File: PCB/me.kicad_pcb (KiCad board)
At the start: 2 copper layers, 107.9 x 100 mm, 16 parts, among them M1 Motor_DC, Q1 AO3400A, SW1 SW_Push, SW2 SW_Push, SW3 SW_Push, SW4 SW_Push, SW5 SW_Push, SW6 SW_Push, U1 XIAO-RP2040-DIP

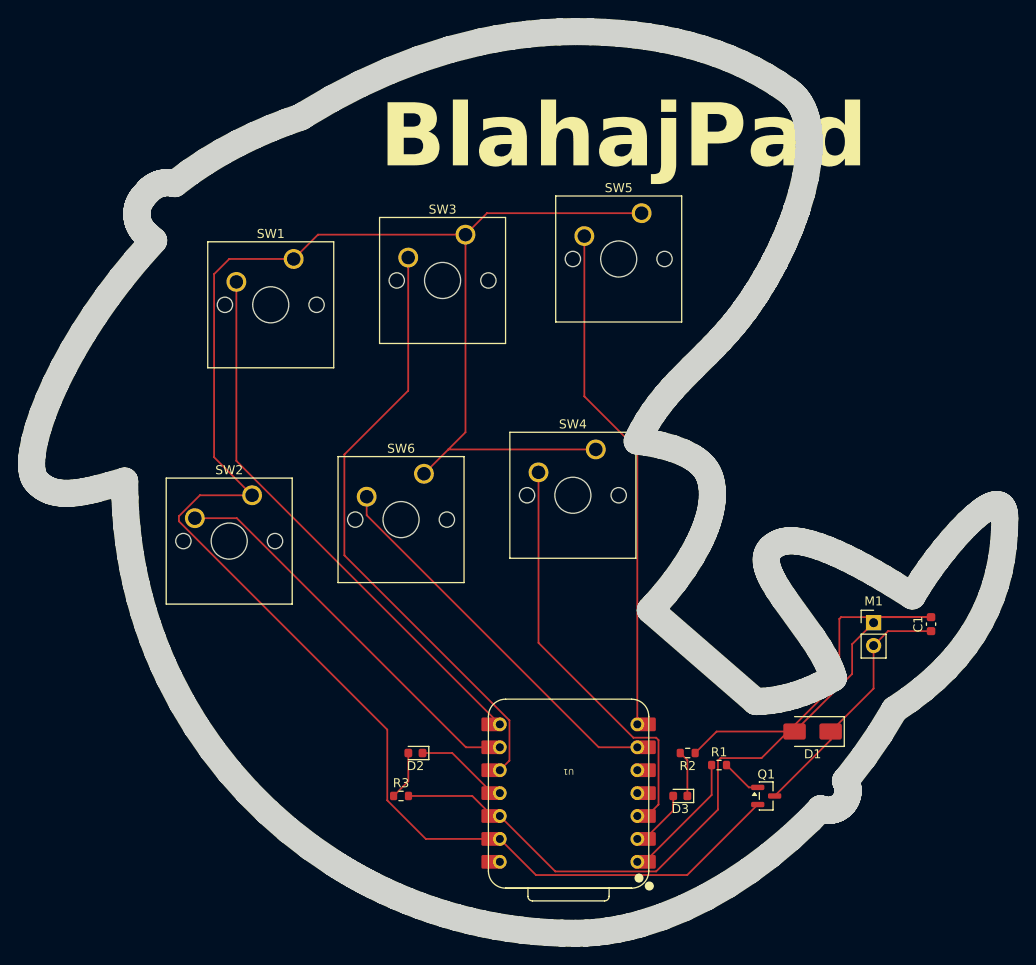
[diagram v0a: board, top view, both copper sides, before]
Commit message: everything's smaller now
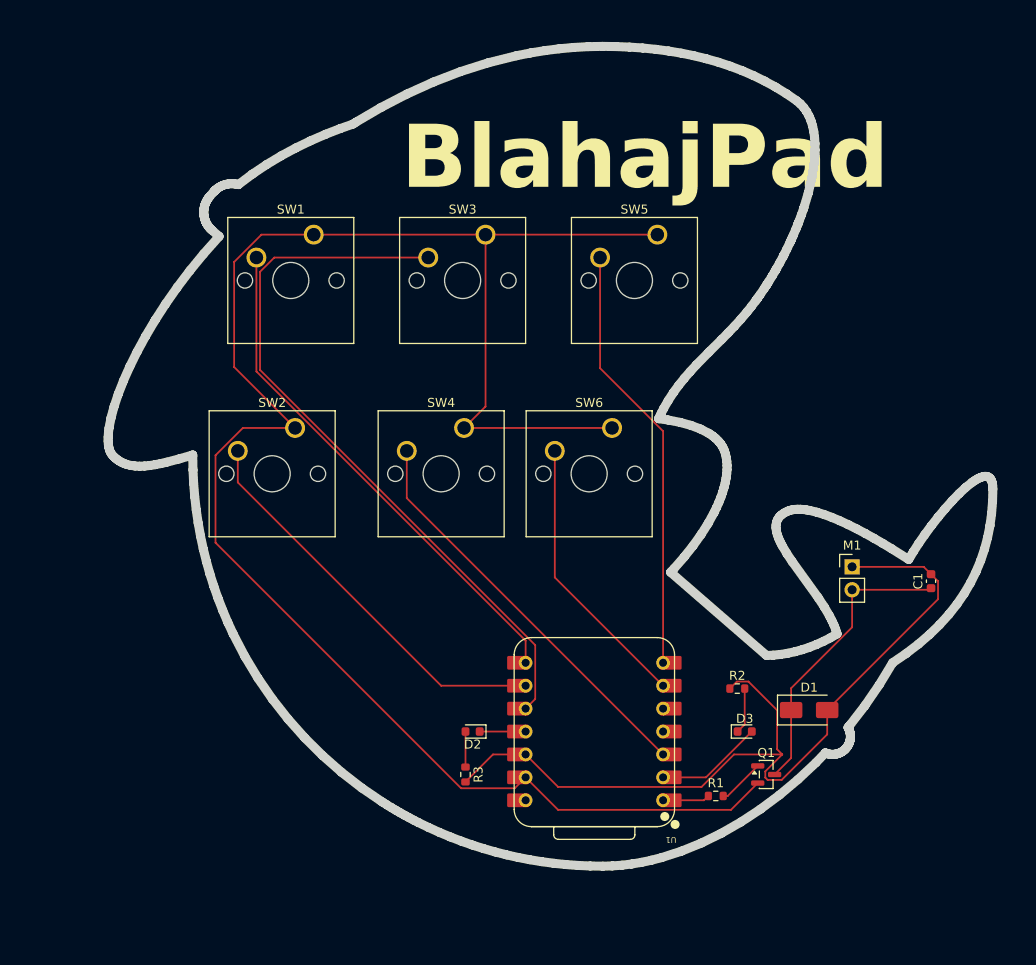
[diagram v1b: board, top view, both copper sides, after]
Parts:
- moved SW6 21.5 mm to (161.5, 92.6)
- moved SW4 14.8 mm to (145.1, 92.6)
- moved D3 10.1 mm to (176.2, 126.2), turned to 0 degrees
- moved R2 9.01 mm to (175.4, 121.4), turned to 0 degrees
- moved SW2 8.85 mm to (126.4, 92.6)
- moved R3 7.53 mm to (145.3, 131.0), turned to -90 degrees
- moved U1 7.40 mm to (159.5, 126.2)
- moved D2 6.77 mm to (146.0, 126.2)
- moved M1 6.63 mm to (188.1, 108.0)
- moved C1 4.76 mm to (196.9, 109.5)
- moved SW1 3.50 mm to (128.4, 71.1)
- moved R1 3.45 mm to (173.0, 133.3)
- moved SW5 2.95 mm to (166.5, 71.1)
- moved D1 2.41 mm to (183.4, 123.8), turned to 0 degrees
- moved Q1 2.38 mm to (178.6, 131.0)
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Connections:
- U1 pad 14: +5V -> unconnected-(U1-VBUS-Pad14)_1
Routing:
- net +3.3V: track 113.7 -> 96.0 mm
- net GND: track 219.1 -> 202.6 mm
- net Net-(U1-GPIO4/MISO): track 68.4 -> 80.8 mm
- net Net-(U1-GPIO7/SCL): track 42.7 -> 31.0 mm
- net Net-(U1-GPIO0/TX): track 59.3 -> 47.8 mm
- net Net-(U1-GPIO26/ADC0/A0): track 13.8 -> 5.21 mm
- net Net-(D3-A): track 6.06 -> 11.1 mm
- net Net-(D1-K): track 28.2 -> 32.9 mm
- net Net-(D2-K): track 9.58 -> 5.09 mm
- net Net-(U1-GPIO1/RX): track 61.2 -> 57.3 mm
- net Net-(D2-A): track 5.44 -> 3.94 mm
- net Net-(U1-GPIO28/ADC2/A2): track 46.7 -> 45.4 mm
- net Net-(Q1-G): track 4.49 -> 5.20 mm
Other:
- board size 107.9 x 100 mm -> 98.1 x 90.9 mm

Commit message: turns out im sped
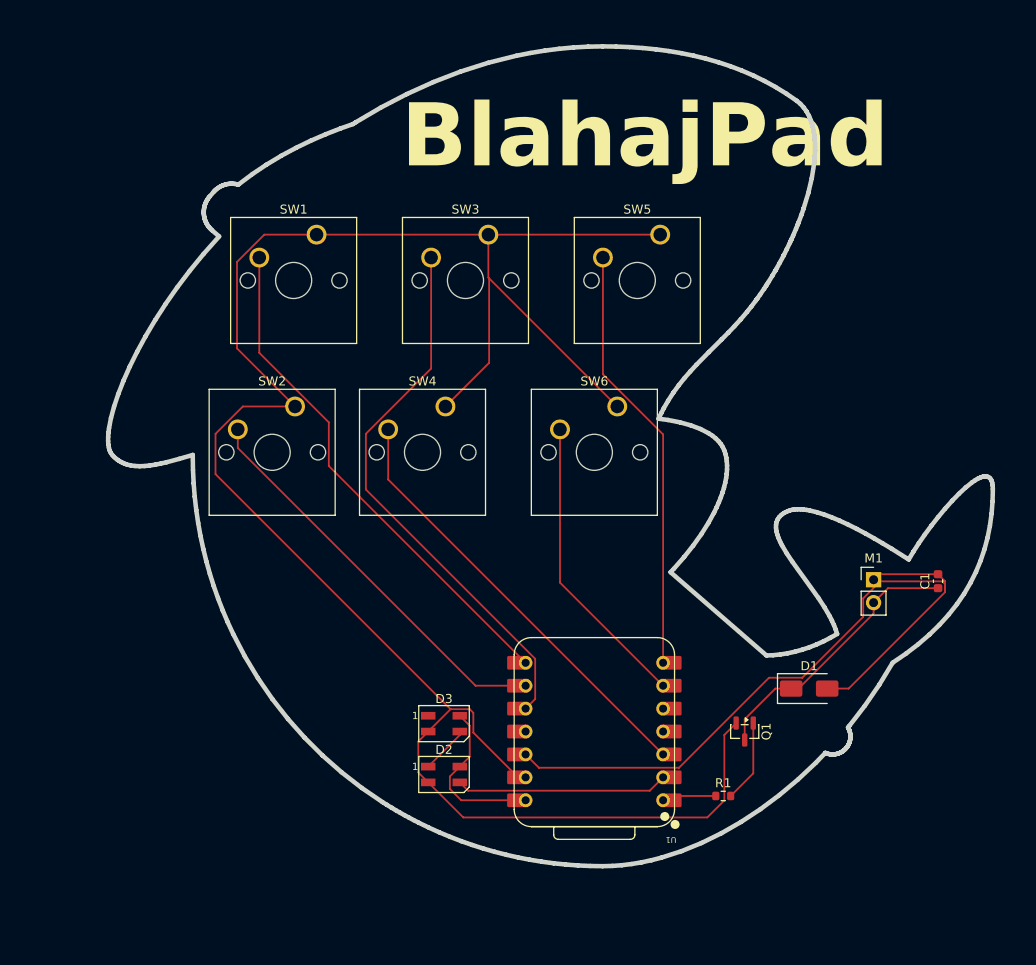
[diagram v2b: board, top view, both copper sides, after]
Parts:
- removed R2, R3: 1kΩ, Resistor_SMD:R_0603_1608Metric
- D2, D3: value LED -> SK6812MINI; footprint LED_SMD:LED_0603_1608Metric -> LED_SMD:LED_SK6812MINI_PLCC4_3.5x3.5mm_P1.75mm
- moved D3 33.3 mm to (142.9, 125.3)
- moved D2 5.72 mm to (142.9, 131.0), turned to 0 degrees
- moved Q1 5.32 mm to (176.2, 126.2), turned to -90 degrees
- moved SW4 3.15 mm to (143.0, 90.2)
- moved M1 2.78 mm to (190.5, 109.4)
- moved SW6 2.45 mm to (162.1, 90.2)
- moved D1 2.38 mm to (183.4, 121.4)
- moved SW2 2.38 mm to (126.4, 90.2)
- moved R1 0.83 mm to (173.8, 133.3)
- moved C1 0.78 mm to (197.6, 109.5)
- moved SW1 0.32 mm to (128.7, 71.1)
- moved SW3 0.32 mm to (147.8, 71.1)
- moved SW5 0.32 mm to (166.8, 71.1)
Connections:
- D2 pad 1: Net-(D2-K) -> Net-(D2-DOUT)
- D2 pad 2: Net-(D2-A) -> GND
- D3 pad 1: Net-(D3-K) -> unconnected-(D3-DOUT-Pad1)
- D3 pad 2: Net-(D3-A) -> GND
- U1 pad 11: Net-(D2-K) -> unconnected-(U1-GPIO3/MOSI-Pad11)_1
- U1 pad 14: unconnected-(U1-VBUS-Pad14)_1 -> +5V
- U1 pad 2: Net-(D3-A) -> Net-(D2-DIN)
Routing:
- net GND: track 202.6 -> 226.6 mm
- net Net-(D2-DIN): track 0.00 -> 23.5 mm
- net Net-(U1-GPIO4/MISO): track 80.8 -> 61.2 mm
- net +5V: track 0.00 -> 18.4 mm
- net Net-(D3-A): track 11.1 -> 0.00 mm
- net +3.3V: track 96.0 -> 85.1 mm
- net Net-(D2-DOUT): track 0.00 -> 5.34 mm
- net Net-(D2-K): track 5.09 -> 0.00 mm
- net Net-(D3-K): track 5.09 -> 0.00 mm
- net Net-(D2-A): track 3.94 -> 0.00 mm
- net Net-(Q1-G): track 5.20 -> 9.12 mm
- net Net-(U1-GPIO28/ADC2/A2): track 45.4 -> 48.7 mm
- net Net-(D1-K): track 32.9 -> 30.5 mm
- net Net-(U1-GPIO7/SCL): track 31.0 -> 33.2 mm
- net Net-(U1-GPIO26/ADC0/A0): track 5.21 -> 6.04 mm
